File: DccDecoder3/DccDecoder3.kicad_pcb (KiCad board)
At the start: 2 copper layers, 94 x 55.9 mm, 33 parts, among them J1 PAD, J10 GND, J2 PAD, J3 0, J4 1, J5 2, J6 3, J7 +V, J8 M_OUT_B, J9 M_OUT_A, Q1 DMG2305UX-7, Q2 2N7002K, Q3 2N7002K, Q4 2N7002K, Q5 2N7002K, Q6 2N7002K, SW1 SW_Push, U1 AP7384-33Y, U2 Pico_RaspberryPico, U3 BDR6133

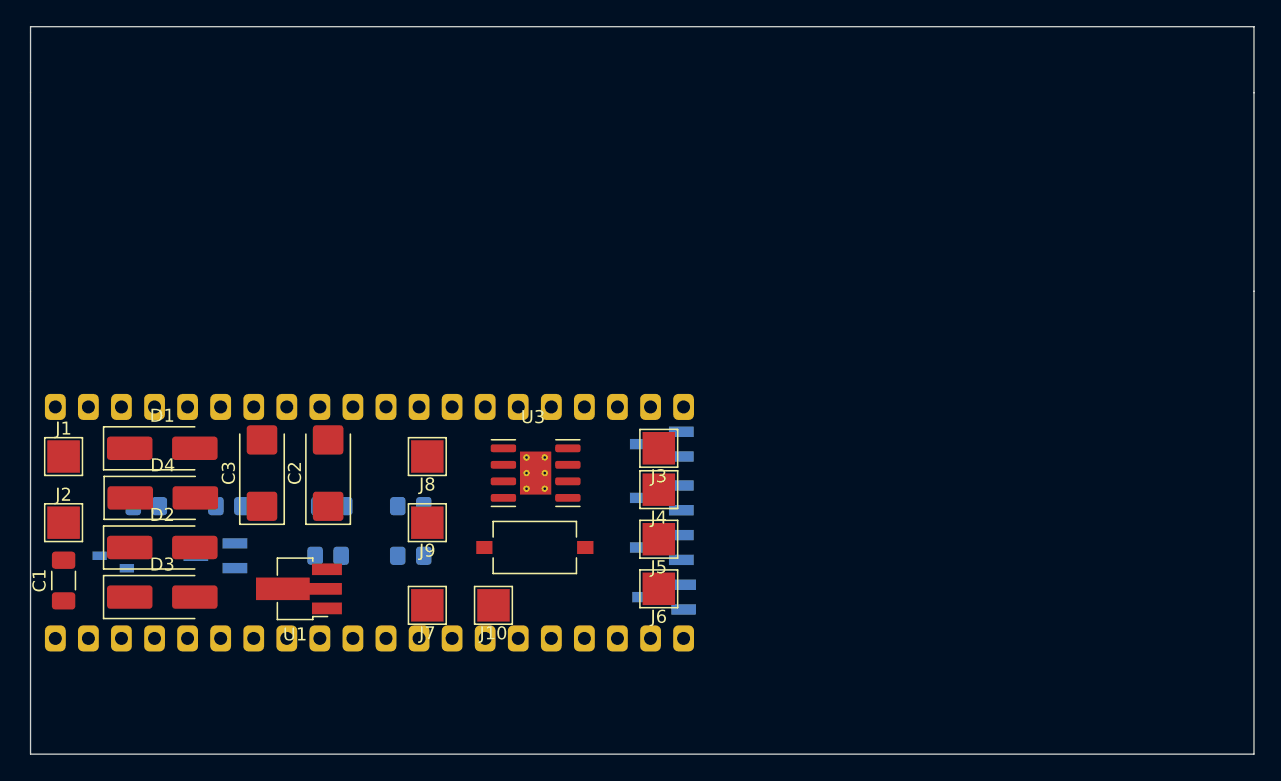
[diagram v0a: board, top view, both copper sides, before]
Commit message: 20/01/25 19:41 Arrakis.local
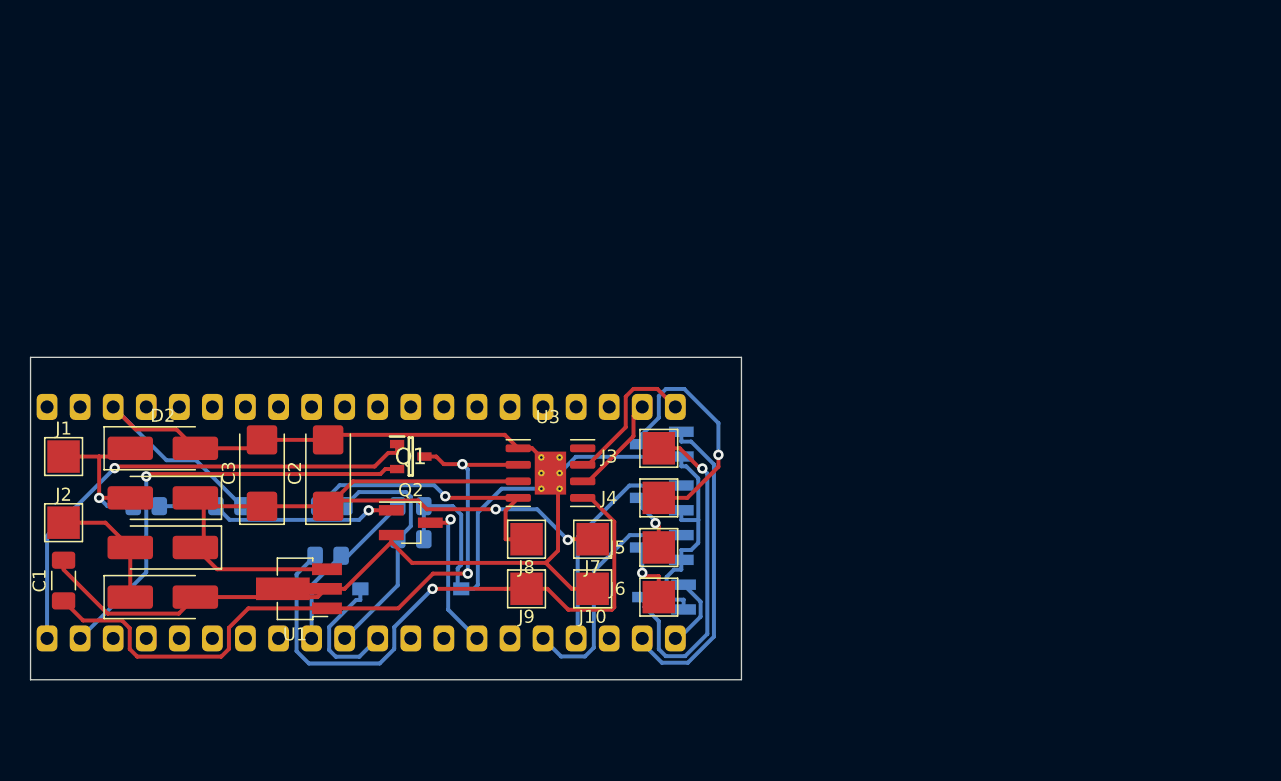
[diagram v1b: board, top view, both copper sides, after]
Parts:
- Q1, Q2: moved to F.Cu
- SW1: moved to B.Cu
- moved Q1 24.1 mm to (128.3, 61.0), turned to 0 degrees
- moved Q2 15.2 mm to (128.3, 66.0), turned to 0 degrees
- moved J7 13.7 mm to (142.2, 67.3)
- moved SW1 10.0 mm to (128.3, 71.1)
- moved J8 9.92 mm to (137.2, 67.3)
- moved J9 9.16 mm to (137.2, 71.1)
- moved J10 7.73 mm to (142.2, 71.1)
- moved D2 7.62 mm to (109.2, 60.3)
- moved D1 3.81 mm to (109.2, 64.1), turned to 180 degrees
- moved D4 3.81 mm to (109.2, 67.9), turned to 180 degrees
- moved R4 1.27 mm to (128.3, 67.3)
- moved U3 1.14 mm to (139.0, 62.2)
- moved J4 0.64 mm to (147.3, 64.1)
- moved U2 0.64 mm to (100.3, 57.1)
- moved J5 0.63 mm to (147.3, 67.9)
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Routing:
- net GND: track 0.00 -> 159.9 mm
- net +V: track 0.00 -> 61.9 mm, vias 0 -> 2
- net +3V3: track 0.00 -> 53.4 mm, vias 0 -> 2
- net /MOTOR_OUT_B: track 0.00 -> 46.6 mm, vias 0 -> 1
- net Net-(U2-VBUS): track 0.00 -> 38.1 mm, vias 0 -> 1
- net /VSYS: track 0.00 -> 34.1 mm, vias 0 -> 1
- net Net-(J3-Pin_1): track 0.00 -> 26.0 mm, vias 0 -> 1
- net /GPIO17: track 0.00 -> 24.5 mm
- net /MOTOR_OUT_A: track 0.00 -> 21.6 mm, vias 0 -> 1
- net Net-(J4-Pin_1): track 0.00 -> 19.0 mm, vias 0 -> 1
- net /ADC_EMF_A: track 0.00 -> 18.7 mm
- net Net-(Q2-G): track 0.00 -> 18.6 mm, vias 0 -> 1
- net /GPIO19: track 0.00 -> 18.5 mm
- net /GPIO18: track 0.00 -> 17.4 mm
- net Net-(D1-A): track 0.00 -> 13.8 mm, vias 0 -> 1
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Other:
- board size 94 x 55.9 mm -> 54.6 x 24.8 mm
